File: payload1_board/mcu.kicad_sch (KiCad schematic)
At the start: 8 parts, among them U1 ATSAMD21G18A-AF

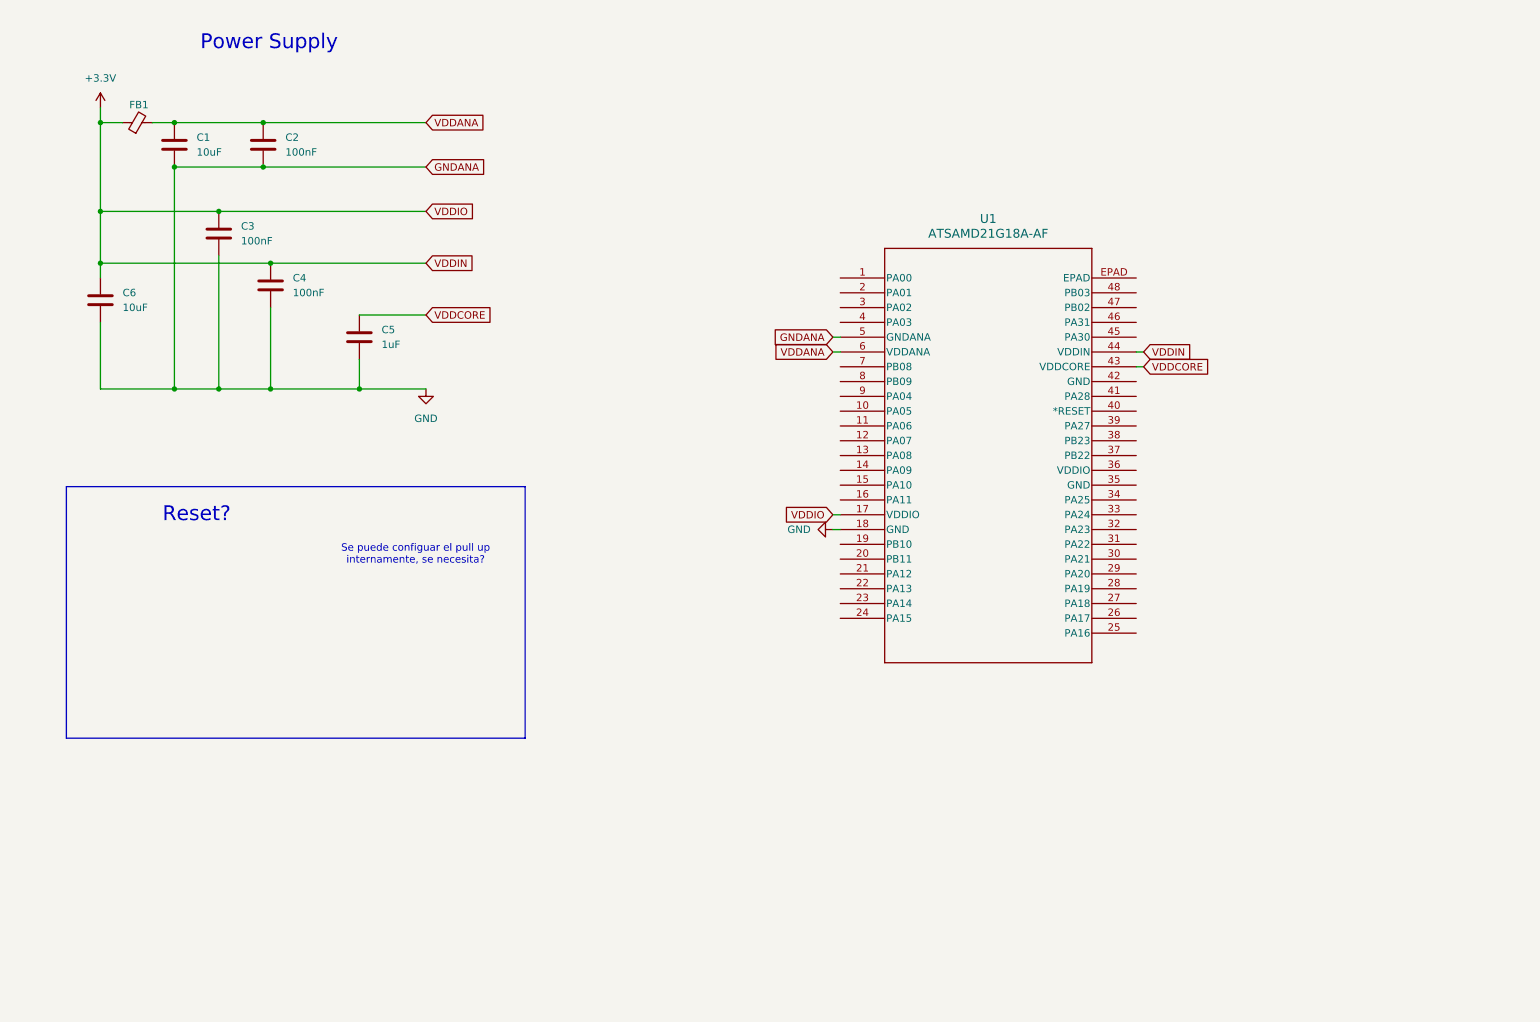
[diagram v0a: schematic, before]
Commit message: Update schematic
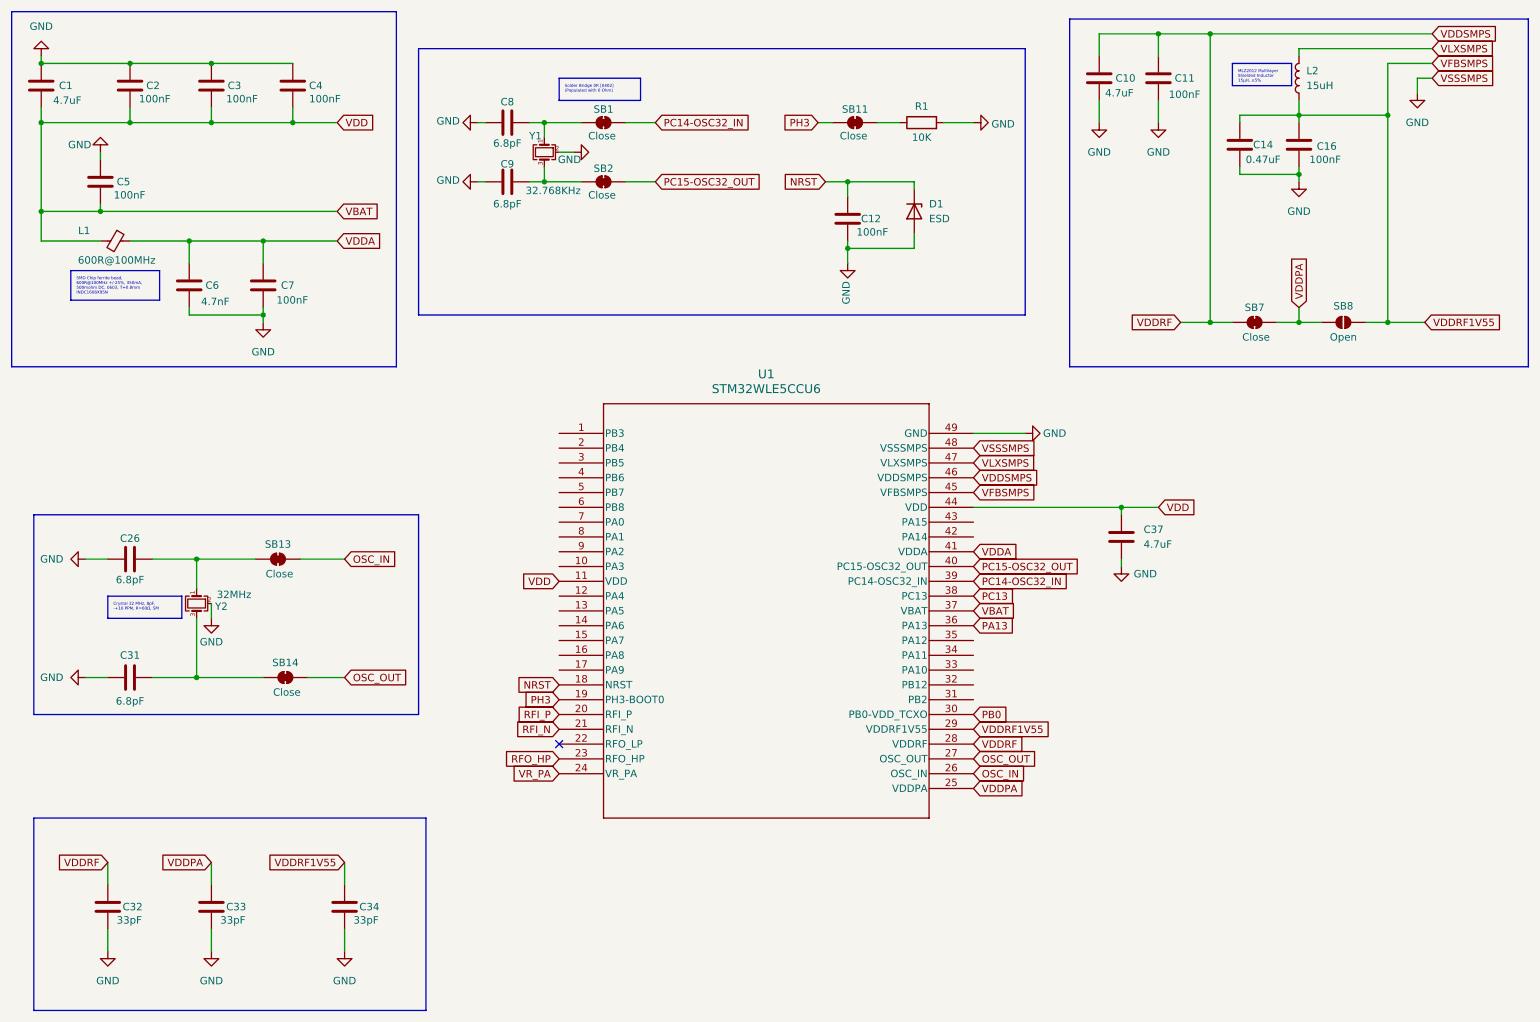
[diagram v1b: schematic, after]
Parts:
- removed FB1: FerriteBead_Small, symbol Device:FerriteBead_Small
- removed U1: ATSAMD21G18A-AF, symbol SAMD21G18A-AF:ATSAMD21G18A-AF
- added C10, C37: 4.7uF, symbol Device:C
- added C11, C12, C16, C7: 100nF, symbol Device:C
- added C14: 0.47uF, symbol Device:C
- added C26, C31, C8, C9: 6.8pF, symbol Device:C
- added C32, C33, C34: 33pF, symbol Device:C
- added D1: ESD, symbol Diode:ESD5Zxx
- added L1: 600R@100MHz, symbol Device:FerriteBead_Small
- added L2: 15uH, symbol Device:L
- added R1: 10K, symbol Device:R
- added SB1, SB11, SB13, SB14, SB2, SB7: Close, symbol Jumper:SolderJumper_2_Bridged
- added SB8: Open, symbol Jumper:SolderJumper_2_Open
- added U1: STM32WLE5CCU6, UFQFPN48_STM, symbol STM32WLE5:STM32WLE5CCU6
- added Y1: 32.768KHz, symbol Device:Crystal_GND24_Small
- added Y2: 32MHz, symbol Device:Crystal_GND24_Small
- C1: value 10uF -> 4.7uF
- C5: value 1uF -> 100nF
- C6: value 10uF -> 4.7nF
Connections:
- net VDDANA is gone; now on net GND: C1.1, C2.1
- net VDDCORE is gone; now on net GND: C5.1
- net GND: now also C3.1, C4.1, C10.2, C11.2, C12.2, C14.2, C16.2, C26.1, C31.1, C32.2, C33.2, C34.2, C37.2, C7.2, C8.1, C9.1, D1.2 (A), R1.2, U1.48 (VSSSMPS), U1.49 (GND), Y1.2 (G), Y1.4 (G), Y2.2 (G), Y2.4 (G); no longer C1.2, C2.2, C3.2, C4.2, C5.2
- removed net +3.3V: C3.1, C4.1, C6.1
- new net: C26.2, SB13.1 (A), Y2.1
- new net: C9.2, SB2.1 (A), Y1.3
- new net: C31.2, SB14.1 (A), Y2.3
- new net: C8.2, SB1.1 (A), Y1.1
- new net: R1.1, SB11.2 (B)
- new net NRST: C12.1, D1.1 (K), U1.18 (NRST)
- new net OSC_IN: SB13.2 (B), U1.26 (OSC_IN)
- new net OSC_OUT: SB14.2 (B), U1.27 (OSC_OUT)
- new net PA13: U1.36 (PA13)
- new net PB0: U1.30 (PB0-VDD_TCXO)
- new net PC13: U1.38 (PC13)
- new net PC14-OSC32_IN: SB1.2 (B), U1.39 (PC14-OSC32_IN)
- new net PC15-OSC32_OUT: SB2.2 (B), U1.40 (PC15-OSC32_OUT)
- new net PH3: SB11.1 (A), U1.19 (PH3-BOOT0)
- new net RFI_N: U1.21 (RFI_N)
- new net RFI_P: U1.20 (RFI_P)
- new net RFO_HP: U1.23 (RFO_HP)
- new net VBAT: C1.2, C2.2, C3.2, C37.1, C4.2, C5.2, L1.2, U1.11 (VDD), U1.37 (VBAT), U1.44 (VDD)
- new net VDDA: C6.1, C7.1, L1.1, U1.41 (VDDA)
- new net VDDPA: C33.1, SB7.2 (B), SB8.1 (A), U1.25 (VDDPA)
- new net VDDRF: C10.1, C11.1, C32.1, SB7.1 (A), U1.28 (VDDRF), U1.46 (VDDSMPS)
- new net VDDRF1V55: C14.1, C16.1, C34.1, L2.2, SB8.2 (B), U1.29 (VDDRF1V55), U1.45 (VFBSMPS)
- new net VLXSMPS: L2.1, U1.47 (VLXSMPS)
- new net VR_PA: U1.24 (VR_PA)
- no-connect marks 0 -> 1
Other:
- note removed: "Power Supply"
- note removed: "Reset?"
- note removed: "Se puede configuar el pull up internamente, se necesita?"
